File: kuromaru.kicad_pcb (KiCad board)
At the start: 2 copper layers, 119.4 x 95.1 mm, 63 parts, among them J1 USB_C_Receptacle_USB2.0, J102 Serial, J5 Conn_01x02, SW1 SW_Push, SW2 SW_Push, U1 RP2040, U2 GD25Q80CEIGR, U3 XC6210B332MR-G, U4 25LCxxx, Y1 Crystal_GND24

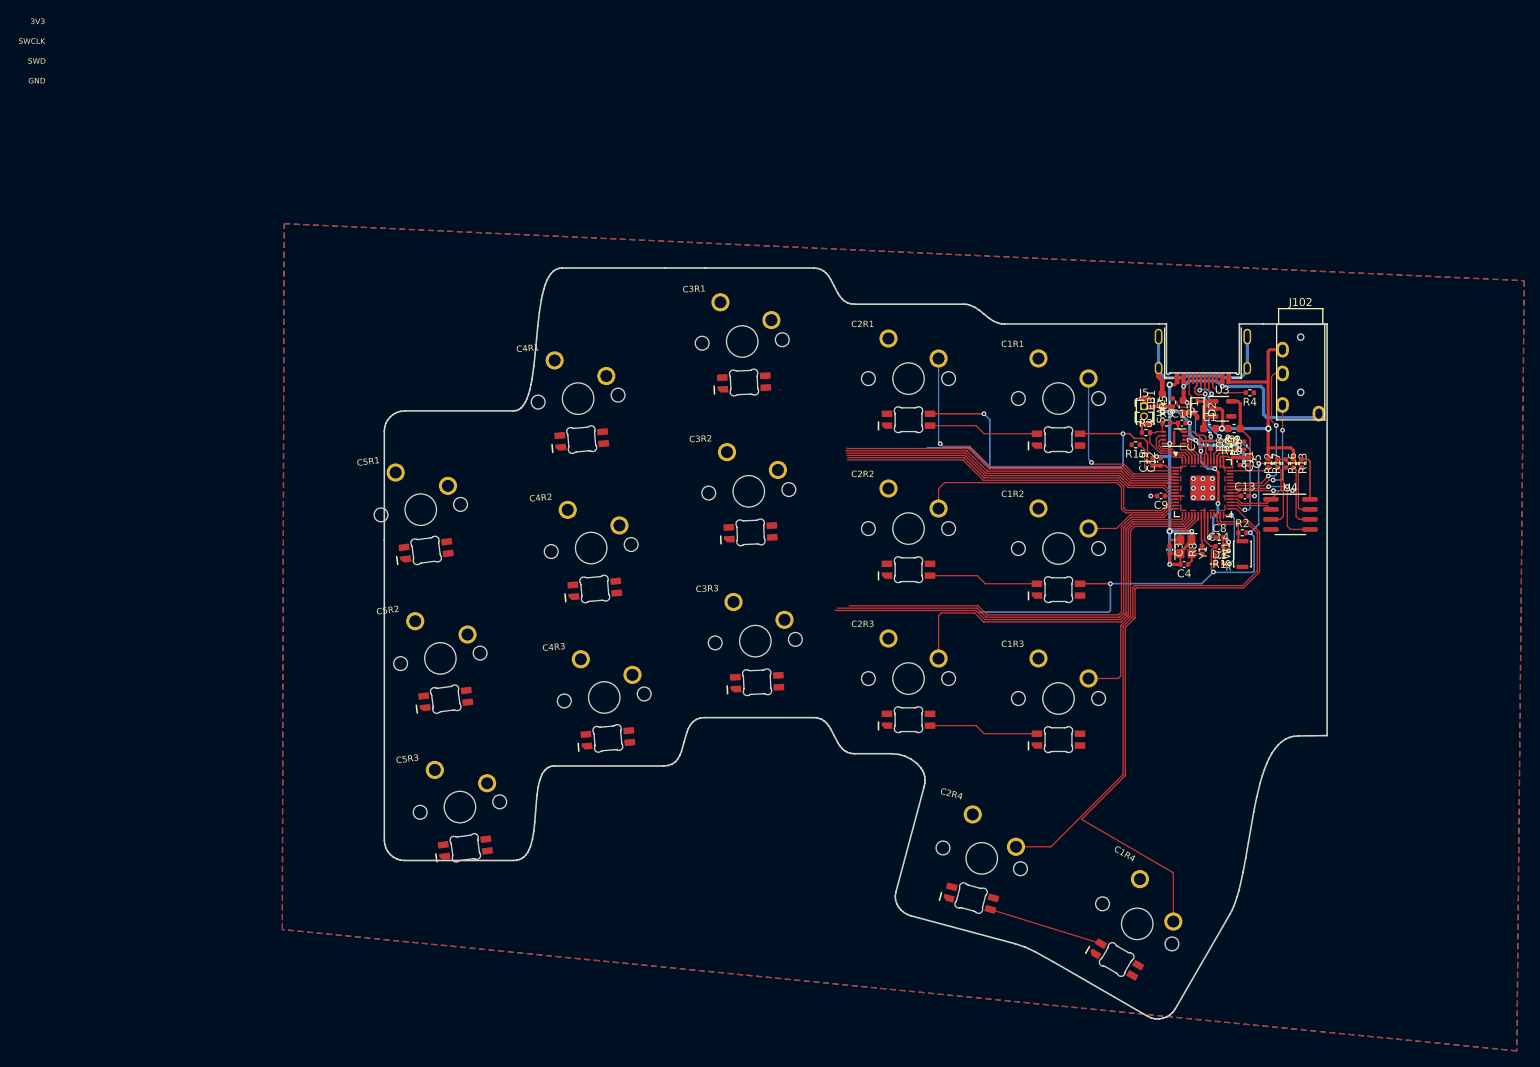
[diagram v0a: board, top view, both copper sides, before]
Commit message: Before messing around with orientation
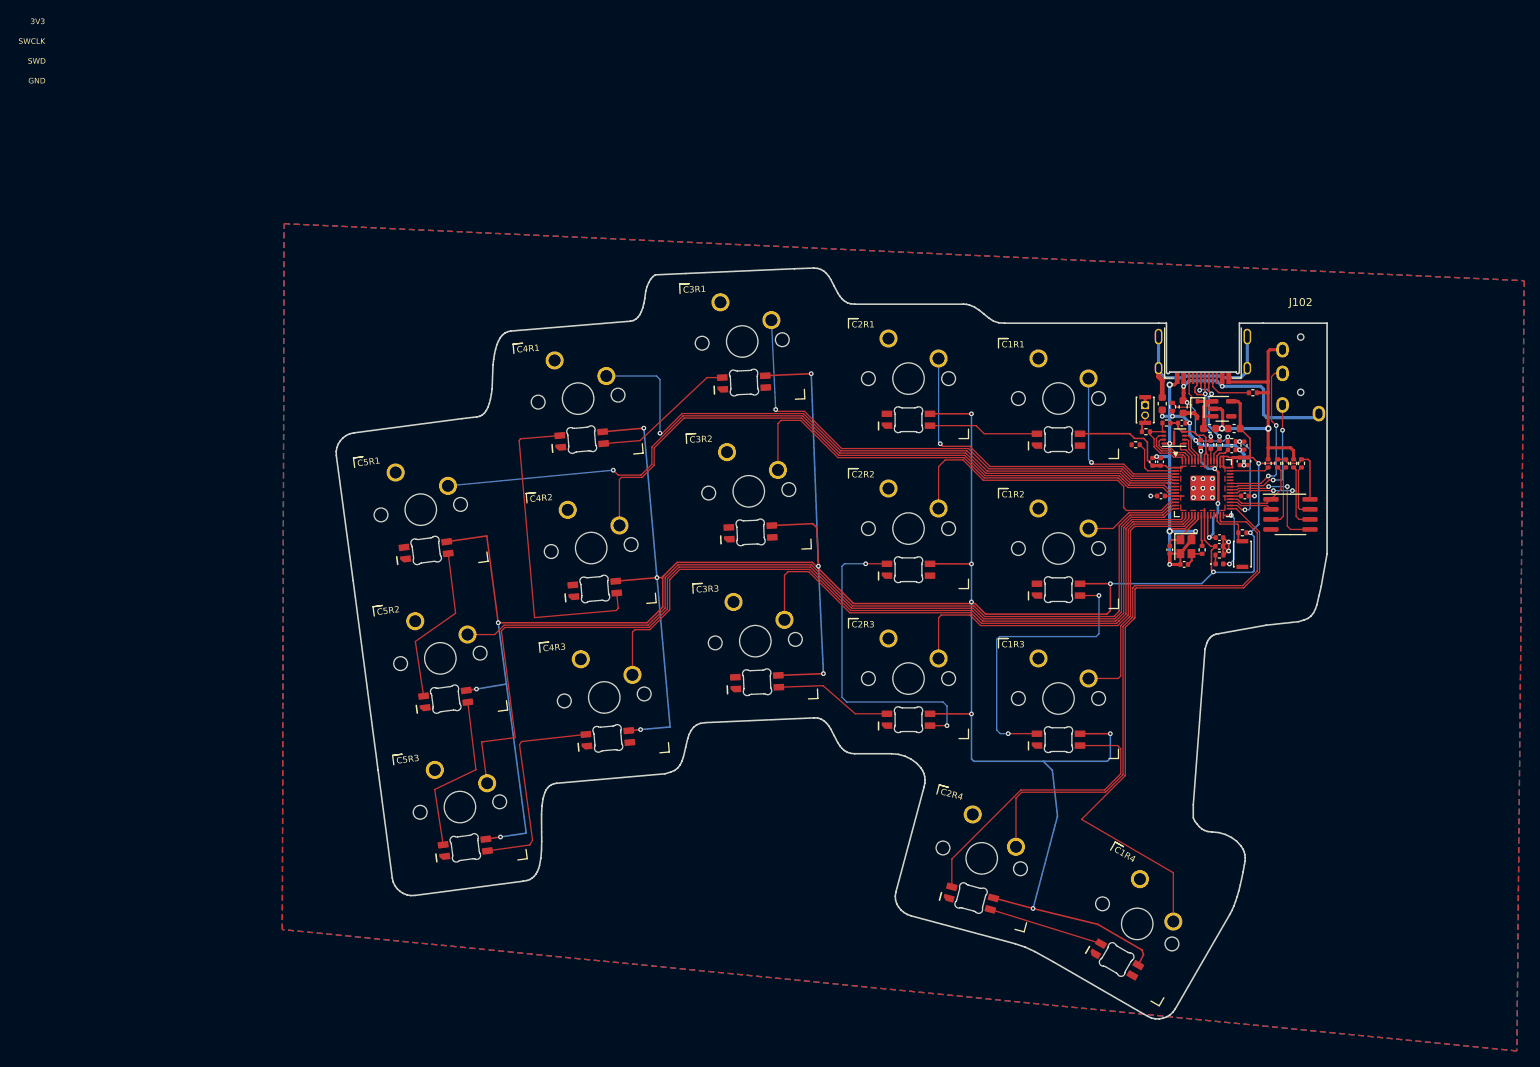
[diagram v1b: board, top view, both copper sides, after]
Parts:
- moved R5 0.55 mm to (143.9, 43.8)
- moved FB1 0.45 mm to (142.6, 43.4)
- moved R4 0.39 mm to (154.1, 42.0)
- moved J5 0.19 mm to (140.4, 43.6)
- moved SW2 0.17 mm to (140.4, 44.2)
- moved R3 0.12 mm to (140.5, 47.0)
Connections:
- C1R1 pad 2: Net-(C1R1-Pad2) -> Net-(C1R2-Pad4)
- C1R2 pad 2: Net-(C1R2-Pad2) -> Net-(C1R3-Pad4)
- C2R2 pad 2: Net-(C1R2-Pad4) -> Net-(C2R1-Pad4)
- C2R2 pad 4: Net-(C2R2-Pad4) -> Net-(C2R3-Pad2)
- C2R3 pad 2: Net-(C1R3-Pad4) -> Net-(C2R3-Pad2)
- C3R1 pad 2: Net-(C2R1-Pad4) -> Net-(C3R2-Pad4)
- C3R2 pad 2: Net-(C2R2-Pad4) -> Net-(C3R3-Pad4)
- C4R1 pad 4: Net-(C4R1-Pad4) -> Net-(C4R2-Pad2)
- C4R2 pad 2: Net-(C3R2-Pad4) -> Net-(C4R2-Pad2)
- C4R3 pad 2: Net-(C3R3-Pad4) -> Net-(C4R2-Pad4)
- C5R1 pad 2: Net-(C4R1-Pad4) -> Net-(C5R2-Pad4)
- C5R2 pad 2: Net-(C4R2-Pad4) -> Net-(C5R3-Pad4)
- C5R2 pad 4: Net-(C1R1-Pad2) -> Net-(C5R2-Pad4)
- C5R3 pad 4: Net-(C1R2-Pad2) -> Net-(C5R3-Pad4)
- U1 pad 11: switch_c3r2 -> switch_c2r2
- U1 pad 12: switch_c2r2 -> switch_c1r2
- U1 pad 13: switch_c1r2 -> switch_c5r2
- U1 pad 8: switch_c5r2 -> switch_c4r2
- U1 pad 9: switch_c4r2 -> switch_c3r2
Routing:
- net +3V3: track 174.6 -> 494.6 mm, vias 6 -> 19
- net switch_c5r3: track 53.7 -> 129.0 mm
- net switch_c5r2: track 43.4 -> 110.5 mm
- net switch_c5r1: track 43.4 -> 100.7 mm, vias 0 -> 1
- net switch_c4r2: track 43.4 -> 84.6 mm
- net Net-(C2R3-Pad2): track 0.00 -> 40.8 mm, vias 0 -> 2
- net Net-(C4R2-Pad2): track 0.00 -> 40.5 mm
- net switch_c4r1: track 43.5 -> 83.8 mm, vias 0 -> 1
- net switch_c4r3: track 56.1 -> 95.4 mm
- net Net-(C1R3-Pad2): track 0.00 -> 37.9 mm
- net Net-(C4R3-Pad4): track 0.00 -> 27.0 mm
- net Net-(C1R3-Pad4): track 14.0 -> 37.3 mm, vias 0 -> 2
- net switch_c3r1: track 43.4 -> 65.7 mm, vias 0 -> 1
- net Net-(C5R3-Pad4): track 0.00 -> 21.5 mm
- net Net-(C5R2-Pad4): track 0.00 -> 20.9 mm
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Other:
- board size 119.4 x 95.1 mm -> 125.5 x 95.1 mm
